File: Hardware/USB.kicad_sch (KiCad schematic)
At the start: 0 parts

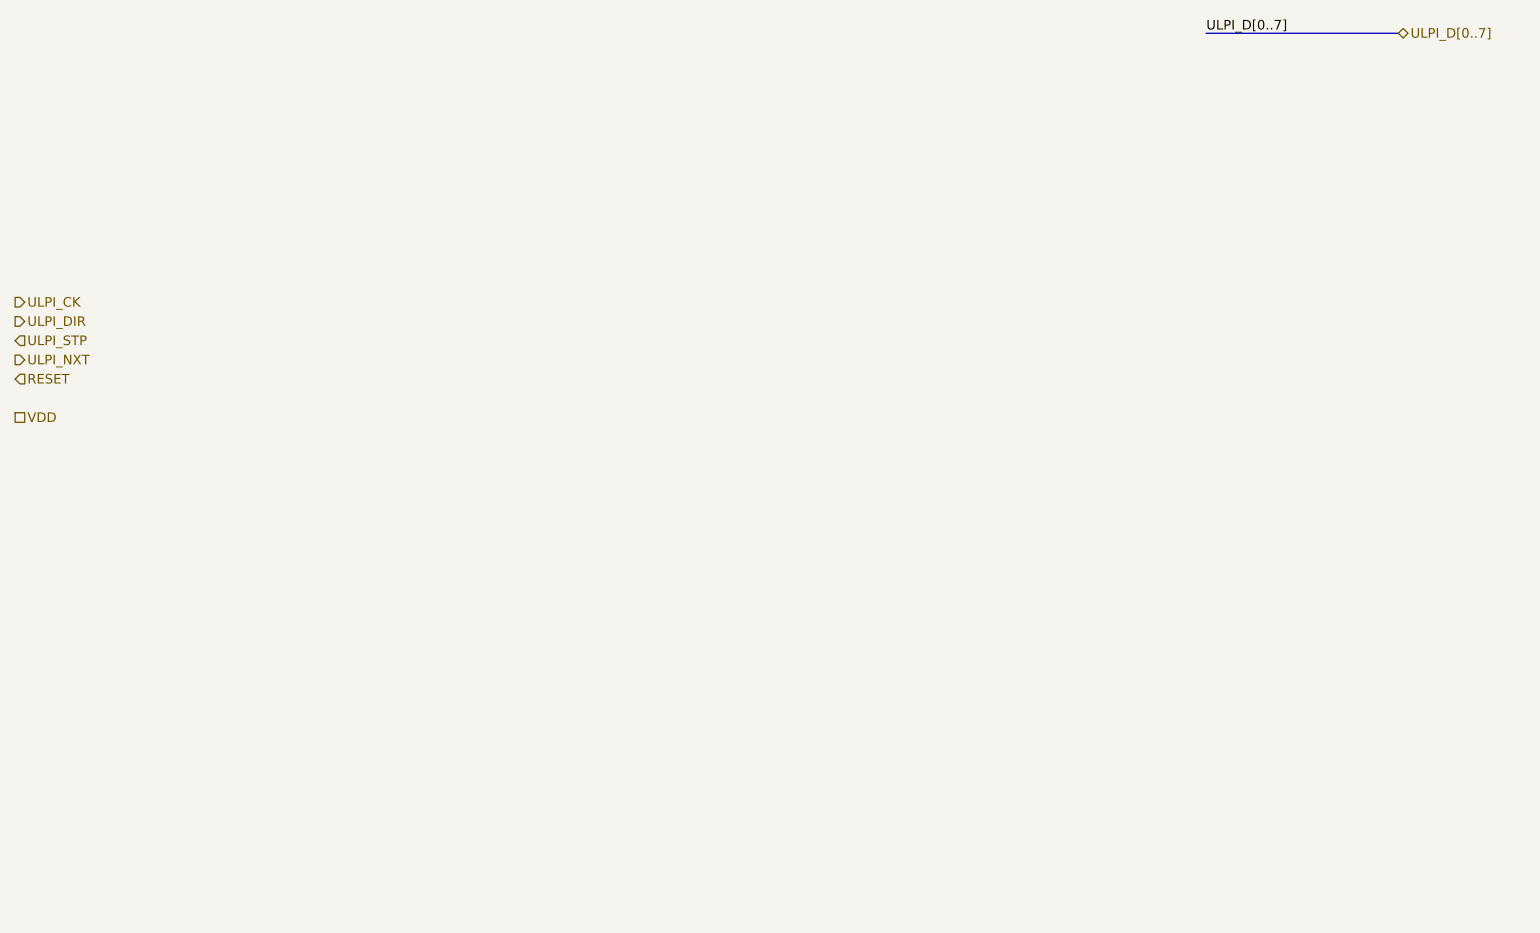
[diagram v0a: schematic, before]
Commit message: Checkpoint
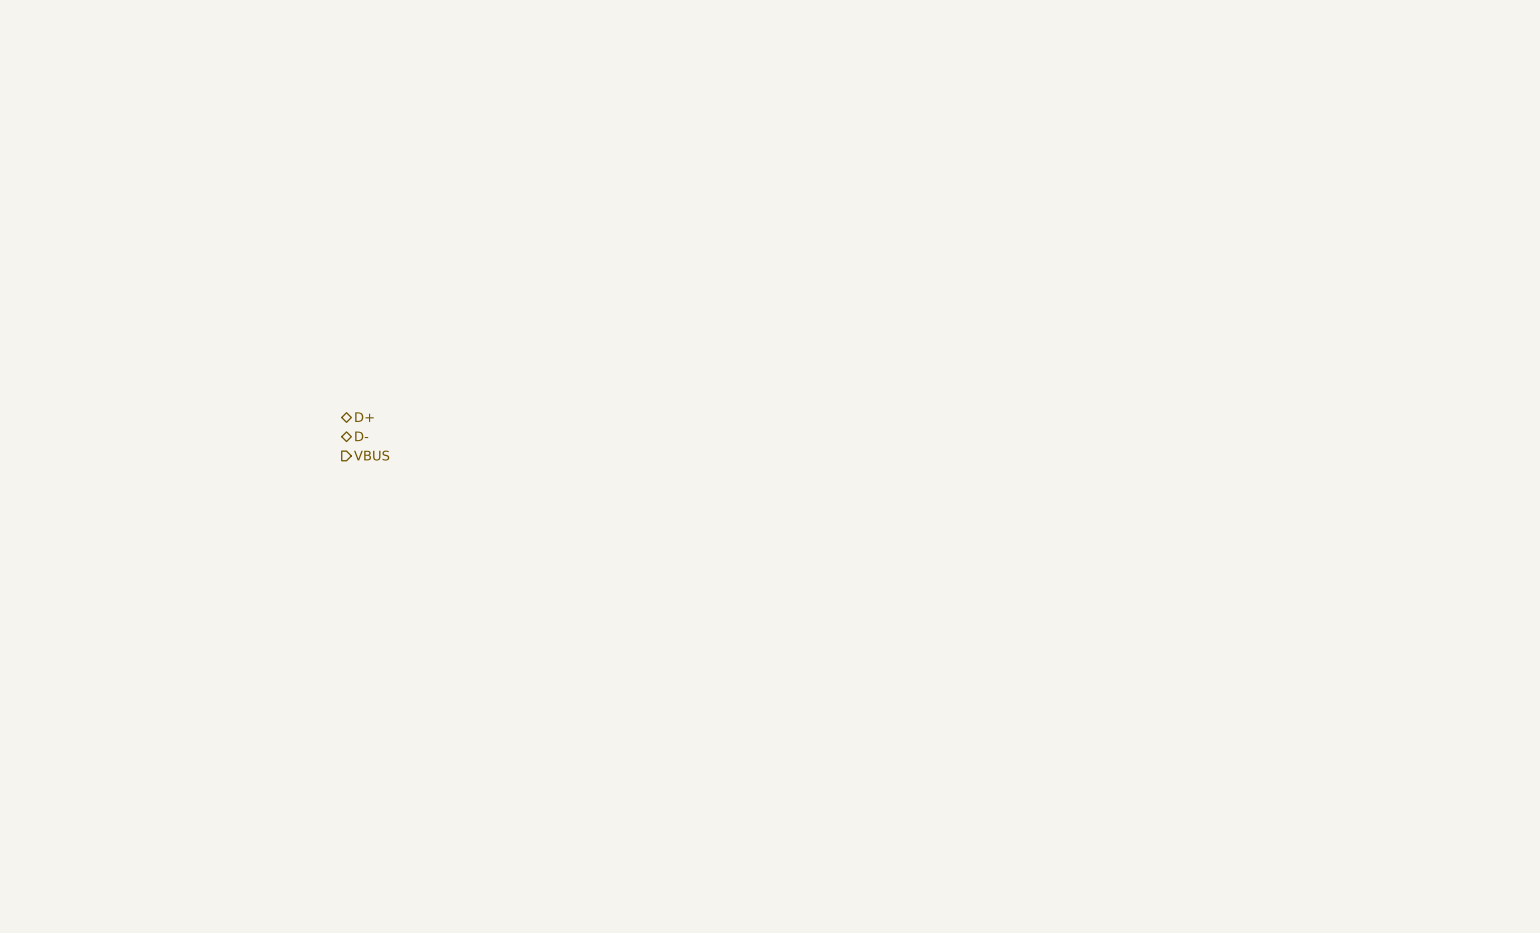
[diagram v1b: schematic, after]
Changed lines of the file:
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@@
 (kicad_sch (version 20230121) (generator eeschema)
   (paper "A4")
-  (bus (pts (xy 241.3 25.4) (xy 266.7 25.4))
-    (stroke (width 0) (type default))
-  )
-  (label "ULPI_D[0..7]" (at 241.3 25.4 0) (fields_autoplaced)
-    (effects (font (size 1.27 1.27)) (justify left bottom))
-  )
-  (hierarchical_label "ULPI_DIR" (shape output) (at 83.82 63.5 0) (fields_autoplaced)
+  (hierarchical_label "VBUS" (shape output) (at 127 81.28 0) (fields_autoplaced)
     (effects (font (size 1.27 1.27)) (justify left))
   )
-  (hierarchical_label "ULPI_D[0..7]" (shape bidirectional) (at 266.7 25.4 0) (fields_autoplaced)
+  (hierarchical_label "D-" (shape bidirectional) (at 127 78.74 0) (fields_autoplaced)
     (effects (font (size 1.27 1.27)) (justify left))
   )
-  (hierarchical_label "ULPI_STP" (shape input) (at 83.82 66.04 0) (fields_autoplaced)
+  (hierarchical_label "D+" (shape bidirectional) (at 127 76.2 0) (fields_autoplaced)
     (effects (font (size 1.27 1.27)) (justify left))
   )
-  (hierarchical_label "VDD" (shape passive) (at 83.82 76.2 0) (fields_autoplaced)
-    (effects (font (size 1.27 1.27)) (justify left))
-  )
-  (hierarchical_label "ULPI_NXT" (shape output) (at 83.82 68.58 0) (fields_autoplaced)
-    (effects (font (size 1.27 1.27)) (justify left))
-  )
-  (hierarchical_label "RESET" (shape input) (at 83.82 71.12 0) (fields_autoplaced)
-    (effects (font (size 1.27 1.27)) (justify left))
-  )
-  (hierarchical_label "ULPI_CK" (shape output) (at 83.82 60.96 0) (fields_autoplaced)
-    (effects (font (size 1.27 1.27)) (justify left))
-  )

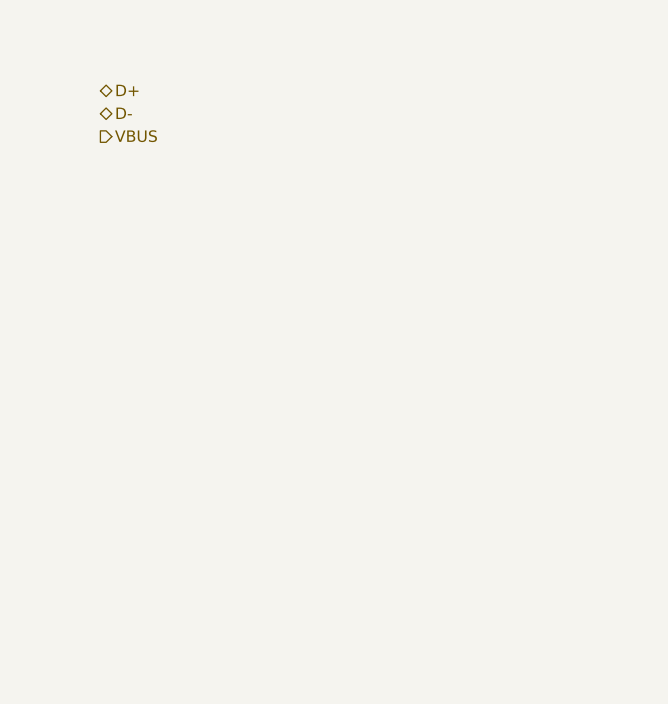
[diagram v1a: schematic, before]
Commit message: Checkpoint
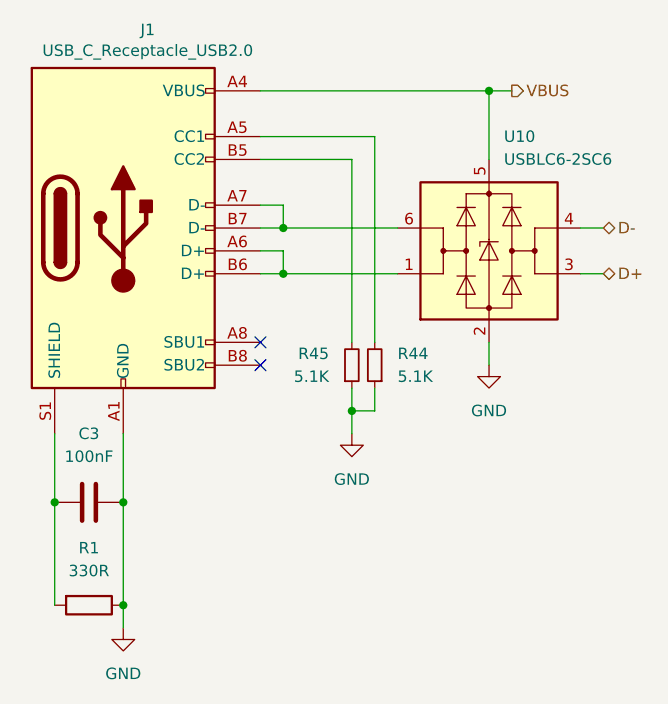
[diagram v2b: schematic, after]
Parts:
- added C3: 100nF, Capacitor_SMD:C_0805_2012Metric, symbol Device:C
- added J1: USB_C_Receptacle_USB2.0, leptunKicadLib:USB4110-GF-A, symbol Connector:USB_C_Receptacle_USB2.0
- added R1: 330R, Resistor_SMD:R_0805_2012Metric, symbol Device:R
- added R44, R45: 5.1K, symbol Device:R_Small
- added U10: USBLC6-2SC6, Package_TO_SOT_SMD:SOT-23-6, symbol Power_Protection:USBLC6-2SC6
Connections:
- net D+: now also U10.3 (I/O2)
- net D-: now also U10.4 (I/O2)
- net VBUS: now also J1.A4 (VBUS), J1.A9 (VBUS), J1.B4 (VBUS), J1.B9 (VBUS), U10.5 (VBUS)
- new net: J1.B5 (CC2), R45.2
- new net: C3.2, J1.S1 (SHIELD), R1.2
- new net: J1.A5 (CC1), R44.2
- new net: J1.A6 (D+), J1.B6 (D+), U10.1 (I/O1)
- new net: J1.A7 (D-), J1.B7 (D-), U10.6 (I/O1)
- new net GND: C3.1, J1.A1 (GND), J1.A12 (GND), J1.B1 (GND), J1.B12 (GND), R1.1, R44.1, R45.1, U10.2 (GND)
- no-connect marks 0 -> 2
